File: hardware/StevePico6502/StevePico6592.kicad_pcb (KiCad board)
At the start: 2 copper layers, 112.4 x 101.6 mm, 35 parts, among them J1 Conn_01x16, J2 Conn_01x16, J3 Conn_02x16_Odd_Even, J4 Conn_01x04, SW1 SW_Push, U1 6551, U2 28C256, U3 GAL16V8, U4 W65C22NxP, U5 CY62256-70PC, U6 74HC00, X1 CXO_DIP14, Y1 1.8432

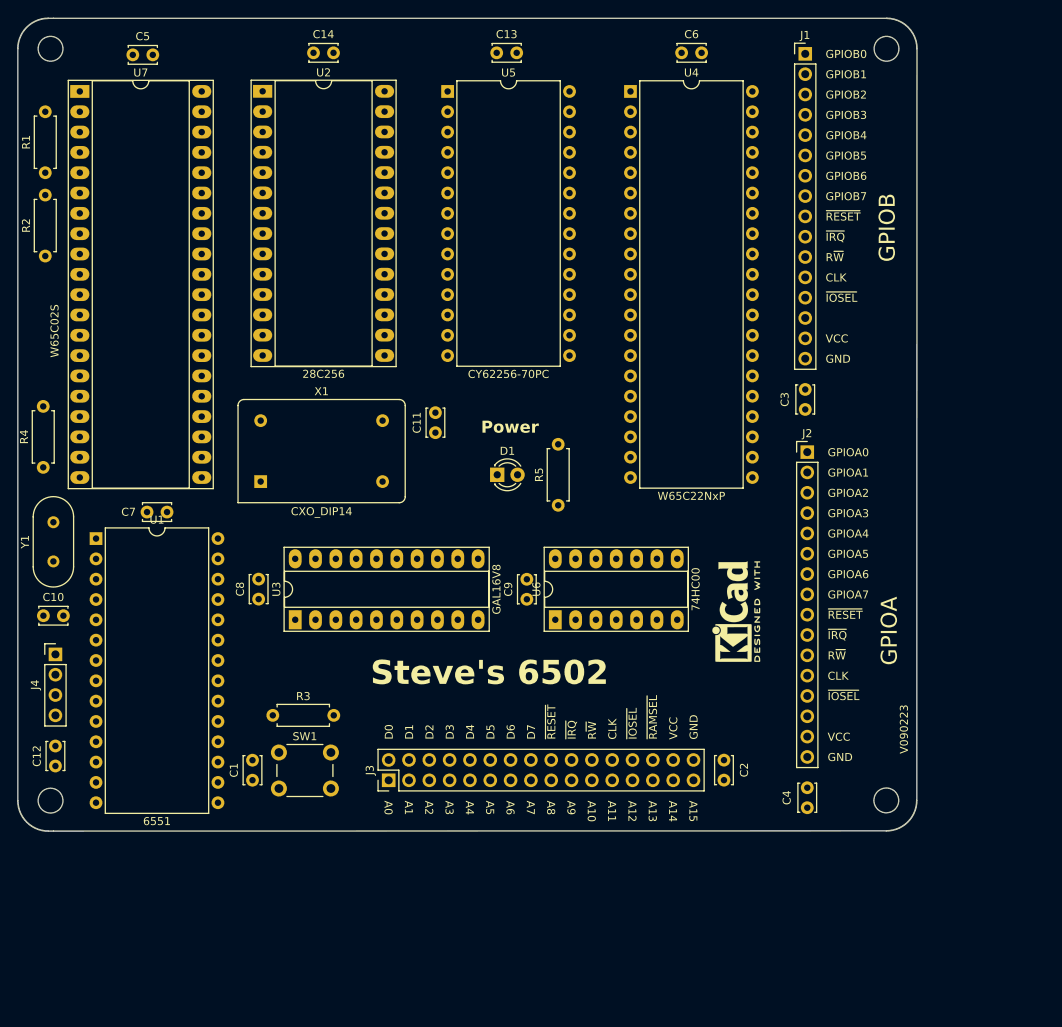
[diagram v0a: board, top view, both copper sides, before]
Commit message: 6502 Rev 2
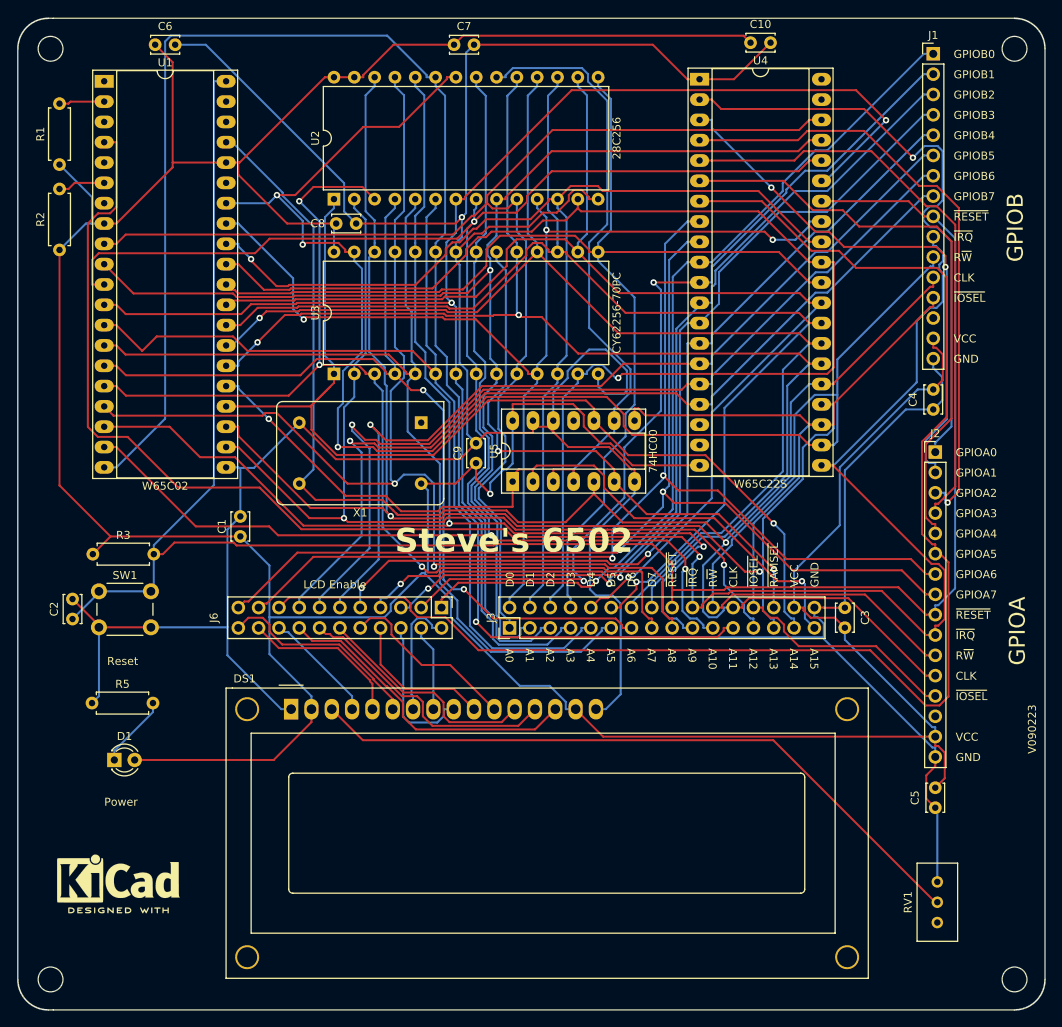
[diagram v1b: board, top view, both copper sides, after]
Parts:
- removed C11, C12, C13, C14: 1uF, Capacitor_THT:C_Disc_D3.4mm_W2.1mm_P2.50mm
- removed the C5 at (63.3, 37.6)
- removed J4: Conn_01x04, Connector_PinHeader_2.54mm:PinHeader_1x04_P2.54mm_Vertical
- removed R4: 1k, Resistor_THT:R_Axial_DIN0207_L6.3mm_D2.5mm_P7.62mm_Horizontal
- removed the REF** at (138.7, 107.2)
- removed U6: 74HC00, Package_DIP:DIP-14_W7.62mm_Socket_LongPads
- removed U7: ~, Package_DIP:DIP-40_W15.24mm_Socket_LongPads
- removed Y1: 1.8432, Crystal:Crystal_HC18-U_Vertical
- added C1: 1uF, Capacitor_THT:C_Disc_D3.4mm_W2.1mm_P2.50mm, F.Cu at (76.7, 97.8)
- added DS1: WC1602A, Display:WC1602A, F.Cu at (83.1, 119.4)
- added J6: Conn_02x11_Odd_Even, Connector_PinHeader_2.54mm:PinHeader_2x11_P2.54mm_Vertical, F.Cu at (101.9, 106.7)
- added REF**: KiCad-Logo2_6mm_SilkScreen, Symbol:KiCad-Logo2_6mm_SilkScreen, F.Cu at (61.5, 140.5)
- added RV1: 10k, Potentiometer_THT:Potentiometer_Bourns_3296W_Vertical, F.Cu at (163.8, 141.0)
- C10: value 30pf -> 1uF
- U1: value 6551 -> W65C02; footprint Package_DIP:DIP-28_W15.24mm -> Package_DIP:DIP-40_W15.24mm_Socket_LongPads
- U2: footprint Package_DIP:DIP-28_W15.24mm_Socket_LongPads -> Package_DIP:DIP-28_W15.24mm
- U3: value GAL16V8 -> CY62256-70PC; footprint Package_DIP:DIP-20_W7.62mm_Socket_LongPads -> Package_DIP:DIP-28_W15.24mm
- U4: value W65C22NxP -> W65C22S; footprint Package_DIP:DIP-40_W15.24mm -> Package_DIP:DIP-40_W15.24mm_Socket_LongPads
- U5: value CY62256-70PC -> 74HC00; footprint Package_DIP:DIP-28_W15.24mm -> Package_DIP:DIP-14_W7.62mm_Socket_LongPads
- moved C10 113.8 mm to (140.5, 36.1)
- moved C7 69.9 mm to (103.4, 36.3)
- moved C6 65.8 mm to (66.1, 36.3)
- moved R5 63.3 mm to (58.2, 118.6), turned to 0 degrees
- moved D1 59.7 mm to (61.0, 125.7)
- moved U1 57.2 mm to (59.7, 40.9)
- moved U5 49.4 mm to (110.7, 90.9), turned to 90 degrees
- moved C8 47.9 mm to (88.7, 58.7), turned to 0 degrees
- moved U3 31.1 mm to (88.4, 77.5)
- moved SW1 30.2 mm to (59.0, 104.6)
- moved C2 30.2 mm to (55.7, 108.1)
- moved R3 30.2 mm to (58.3, 100.0)
- moved J3 24.3 mm to (110.4, 109.2)
- moved C3 24.3 mm to (152.3, 109.2)
- moved X1 21.4 mm to (99.3, 83.6), turned to 180 degrees
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- renumbered C1 to C2, C2 to C3, C3 to C4, C4 to C5
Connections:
- C10 pad 1: Net-(U1-XTAL2) -> VCC
- R1 pad 2: Net-(U7-RDY) -> Net-(U1-RDY)
- R2 pad 2: Net-(U7-NMIB) -> Net-(U1-NMIB)
- U1 pad 1: GND -> unconnected-(U1-VPB-Pad1)
- U1 pad 10: /TXD -> /A1
- U1 pad 11: unconnected-(U1-~{DTR}-Pad11) -> /A2
- U1 pad 12: /RXD -> /A3
- U1 pad 13: /A0 -> /A4
- U1 pad 14: /A1 -> /A5
- U1 pad 15: VCC -> /A6
- U1 pad 16: unconnected-(U1-~{DCD}-Pad16) -> /A7
- U1 pad 17: unconnected-(U1-~{DSR}-Pad17) -> /A8
- U1 pad 18: /D0 -> /A9
- U1 pad 19: /D1 -> /A10
- U1 pad 2: /UARTSEL -> Net-(U1-RDY)
- U1 pad 20: /D2 -> /A11
- U1 pad 21: /D3 -> GND
- U1 pad 22: /D4 -> /A12
- U1 pad 23: /D5 -> /A13
- U1 pad 24: /D6 -> /A14
- U1 pad 25: /D7 -> /A15
- U1 pad 26: unconnected-(U1-~{IRQ}-Pad26) -> /D7
- U1 pad 27: /CLK -> /D6
- U1 pad 28: /R~{W} -> /D5
- U1 pad 3: /~{UARTSEL} -> unconnected-(U1-PHI1O-Pad3)
- U1 pad 4: /~{RESET} -> /~{IRQ}
- U1 pad 6: Net-(U1-XTAL1) -> Net-(U1-NMIB)
- U1 pad 7: Net-(U1-XTAL2) -> unconnected-(U1-SYNC-Pad7)
- U1 pad 8: unconnected-(U1-~{RTS}-Pad8) -> VCC
- U1 pad 9: unconnected-(U1-~{CTS}-Pad9) -> /A0
- U3 pad 1: /A15 -> /A14
- U3 pad 10: GND -> /A0
- U3 pad 11: unconnected-(U3-I10/~{OE}-Pad11) -> /D0
- U3 pad 12: unconnected-(U3-IO8-Pad12) -> /D1
- U3 pad 13: unconnected-(U3-IO7-Pad13) -> /D2
- U3 pad 14: unconnected-(U3-IO6-Pad14) -> GND
- U3 pad 15: unconnected-(U3-IO5-Pad15) -> /D3
- U3 pad 16: /~{UARTSEL} -> /D4
- U3 pad 17: /~{IOSEL} -> /D5
- U3 pad 18: /~{RAMSEL} -> /D6
- U3 pad 19: /~{ROMSEL} -> /D7
- U3 pad 2: /A14 -> /A12
- U3 pad 20: VCC -> /~{RAMSEL}
- U3 pad 3: /A13 -> /A7
- U3 pad 4: /A12 -> /A6
- U3 pad 5: /A11 -> /A5
- U3 pad 6: /A10 -> /A4
- U3 pad 7: /R~{W} -> /A3
- U3 pad 8: /CLK -> /A2
- U3 pad 9: unconnected-(U3-I9-Pad9) -> /A1
- U4 pad 10: /GPIOA0 -> /GPIOB0
- U4 pad 11: /GPIOA1 -> /GPIOB1
- U4 pad 12: /GPIOA2 -> /GPIOB2
- U4 pad 13: /GPIOA3 -> /GPIOB3
- U4 pad 14: /GPIOA4 -> /GPIOB4
- U4 pad 15: /GPIOA5 -> /GPIOB5
- U4 pad 16: /GPIOA6 -> /GPIOB6
- U4 pad 17: /GPIOA7 -> /GPIOB7
- U4 pad 2: /GPIOB0 -> /GPIOA0
- U4 pad 24: /IOSEL -> /A13
- U4 pad 3: /GPIOB1 -> /GPIOA1
- U4 pad 4: /GPIOB2 -> /GPIOA2
- U4 pad 5: /GPIOB3 -> /GPIOA3
- U4 pad 6: /GPIOB4 -> /GPIOA4
- U4 pad 7: /GPIOB5 -> /GPIOA5
- U4 pad 8: /GPIOB6 -> /GPIOA6
- U4 pad 9: /GPIOB7 -> /GPIOA7
- U5 pad 1: /A14 -> /A15
- U5 pad 10: /A0 -> /A14
- U5 pad 11: /D0 -> unconnected-(U5-Pad11)
- U5 pad 12: /D1 -> GND
- U5 pad 13: /D2 -> GND
- U5 pad 14: GND -> VCC
- U5 pad 2: /A12 -> /A15
- U5 pad 3: /A7 -> /~{ROMSEL}
- U5 pad 4: /A6 -> /~{ROMSEL}
- U5 pad 5: /A5 -> /CLK
- U5 pad 6: /A4 -> /~{RAMSEL}
- U5 pad 7: /A3 -> GND
- U5 pad 8: /A2 -> /~{IOSEL}
- U5 pad 9: /A1 -> /~{ROMSEL}
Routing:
- net VCC: track 0.00 -> 489.1 mm, vias 0 -> 1
- net GND: track 0.00 -> 461.3 mm, vias 0 -> 1
- net /~{RESET}: track 0.00 -> 253.4 mm
- net /R~{W}: track 0.00 -> 239.9 mm, vias 0 -> 3
- net /~{IRQ}: track 0.00 -> 230.3 mm, vias 0 -> 1
- net /CLK: track 0.00 -> 200.2 mm, vias 0 -> 1
- net /A11: track 0.00 -> 198.7 mm, vias 0 -> 1
- net /A3: track 0.00 -> 185.8 mm, vias 0 -> 2
- net /GPIOA5: track 0.00 -> 181.5 mm
- net /A2: track 0.00 -> 167.7 mm, vias 0 -> 1
- net /A13: track 0.00 -> 167.7 mm, vias 0 -> 2
- net /D2: track 0.00 -> 163.5 mm, vias 0 -> 1
- net /A0: track 0.00 -> 160.2 mm
- net /A1: track 0.00 -> 158.8 mm, vias 0 -> 1
- net /D4: track 0.00 -> 156.0 mm, vias 0 -> 1
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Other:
- board size 112.4 x 101.6 mm -> 128.4 x 124 mm
- board text added: "LCD Enable"
- board text added: "Reset"
- board text removed: "W65C02S"
